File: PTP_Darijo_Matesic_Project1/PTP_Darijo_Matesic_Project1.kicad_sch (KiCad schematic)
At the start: 3 parts

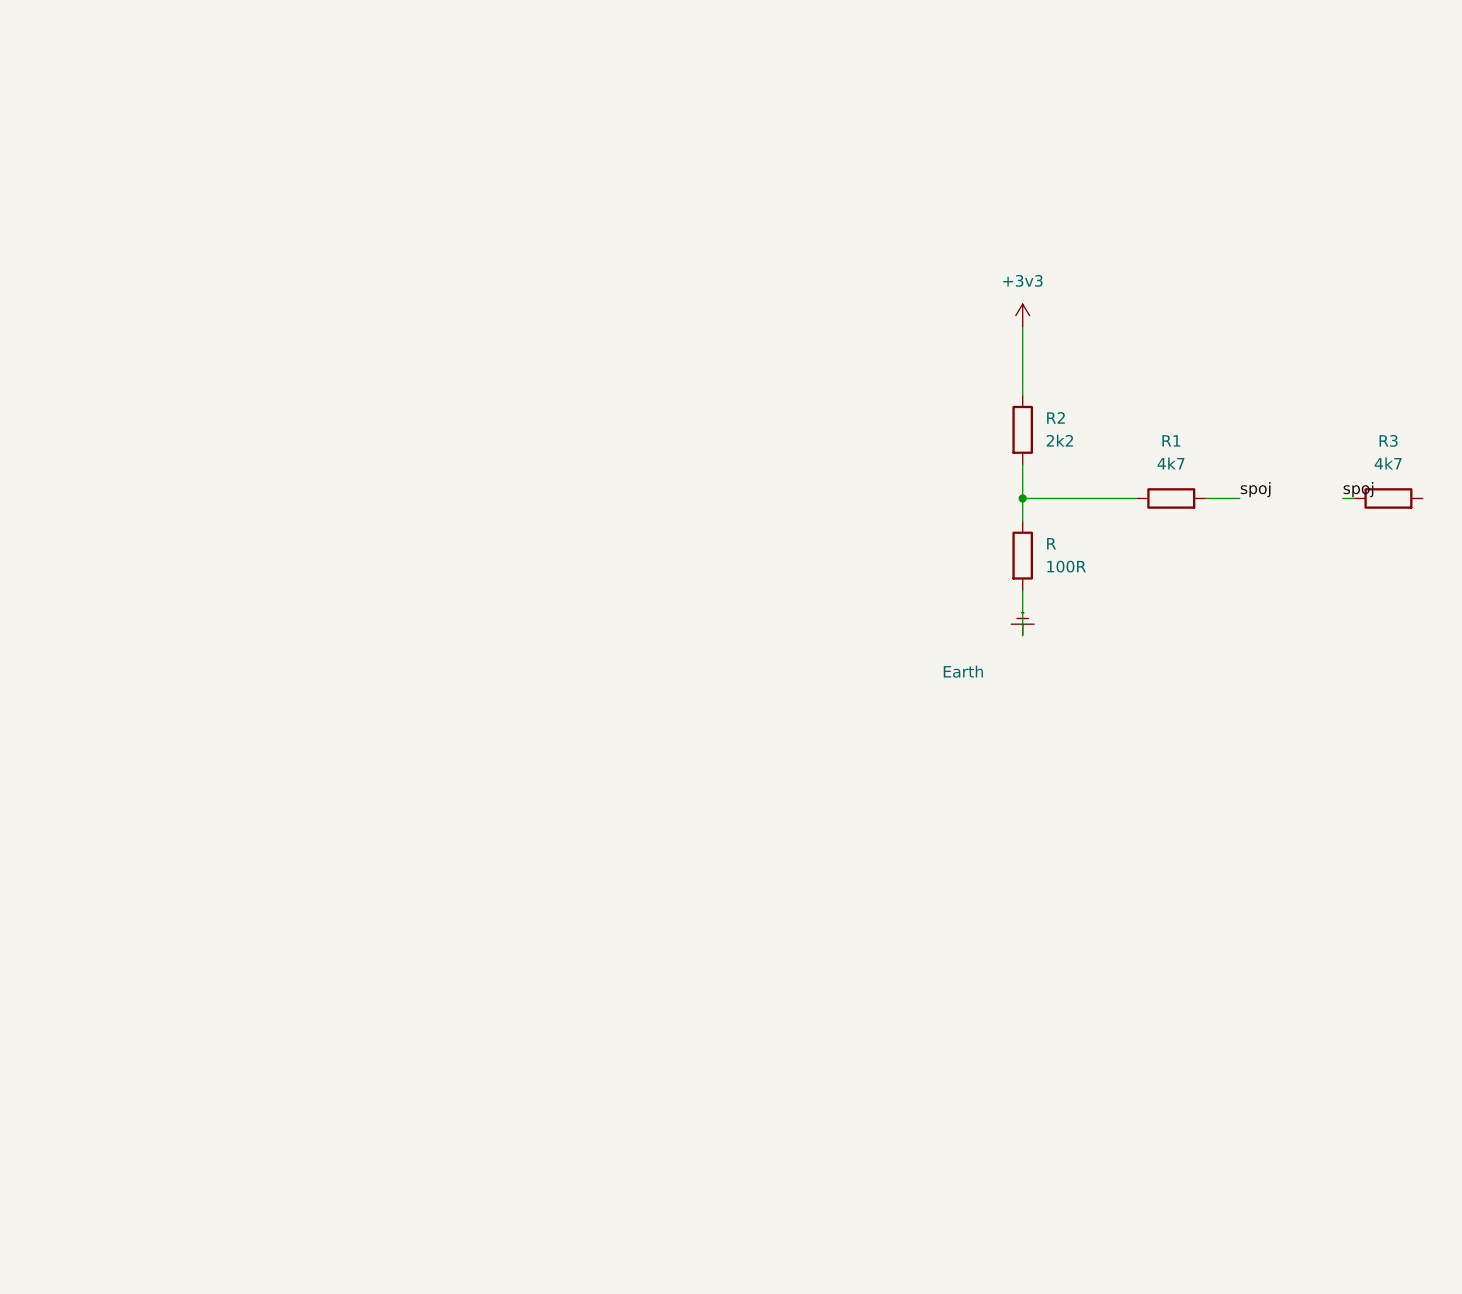
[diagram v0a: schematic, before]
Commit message: A
A
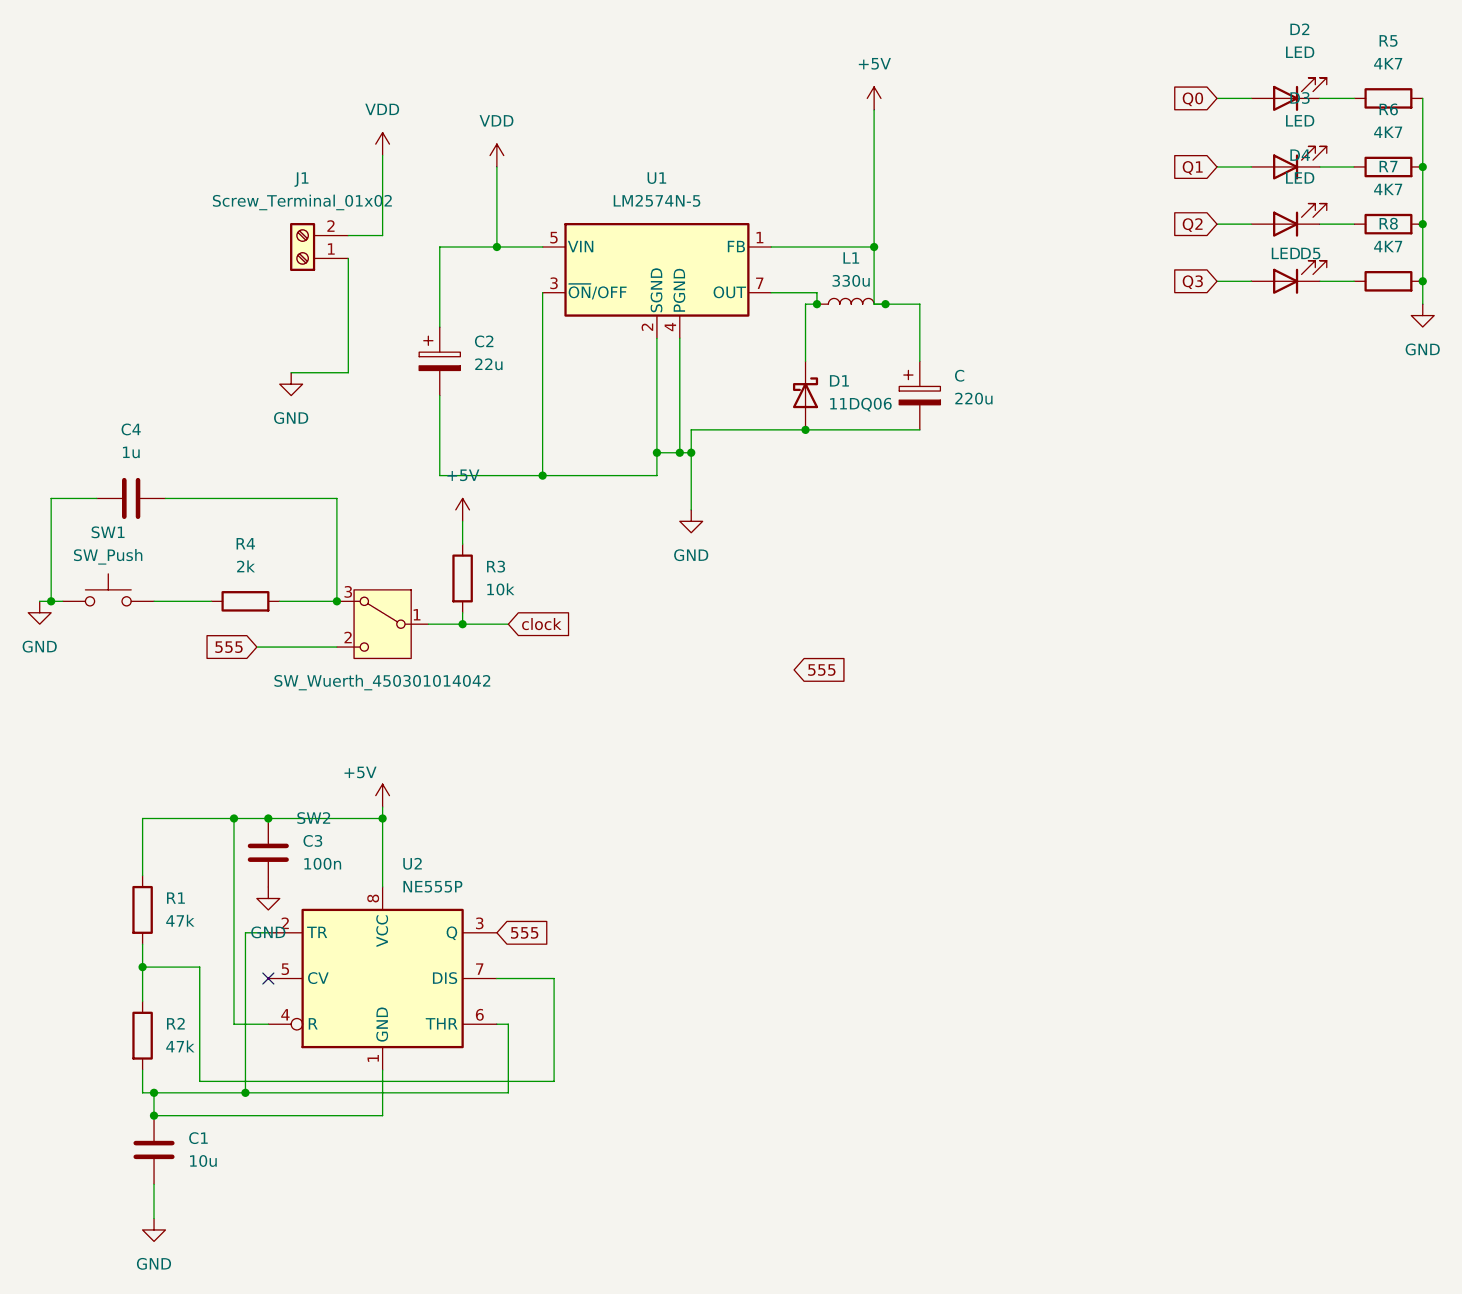
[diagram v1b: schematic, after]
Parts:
- added C: 220u, symbol Device:C_Polarized
- added C1: 10u, symbol Device:C
- added C2: 22u, symbol Device:C_Polarized
- added C3: 100n, symbol Device:C
- added C4: 1u, symbol Device:C
- added D1: 11DQ06, symbol Device:D_Schottky
- added D2, D3, D4, D5: LED, symbol Device:LED
- added J1: Screw_Terminal_01x02, symbol Connector:Screw_Terminal_01x02
- added L1: 330u, symbol Device:L
- added R4: 2k, symbol Device:R
- added R5, R6, R7, R8: 4K7, symbol Device:R
- added SW1: SW_Push, symbol Switch:SW_Push
- added SW2: SW_Wuerth_450301014042, Button_Switch_THT:SW_Slide-03_Wuerth-WS-SLTV_10x2.5x6.4_P2.54mm, symbol Switch:SW_Wuerth_450301014042
- added U1: LM2574N-5, Package_DIP:DIP-8_W7.62mm, symbol Regulator_Switching:LM2574N-5
- added U2: NE555P, Package_DIP:DIP-8_W7.62mm, symbol Timer:NE555P
- R1: value 4k7 -> 47k
- R2: value 2k2 -> 47k
- R3: value 4k7 -> 10k
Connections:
- net Earth is gone; now on an unnamed net: R1.2
- net at R2.2: now also C1.1, U2.1 (GND), U2.2 (TR), U2.6 (THR); no longer R1.1
- net clock: now reaches R3.2
- net clock: now also SW2.1 (B)
- net +3v3: no longer names the net of R2.1
- net +3v3: now also U2.7 (DIS)
- net spoj renamed +5V
- net +5V: now also R1.1, C.1, C3.1, L1.2, U1.1 (FB), U2.4 (R), U2.8 (VCC); no longer R1.2
- new net: C4.2, R4.2, SW2.3 (A)
- new net: D2.1 (K), R5.1
- new net: D4.1 (K), R7.1
- new net: D5.1 (K), R8.1
- new net: D1.1 (K), L1.1, U1.7 (OUT)
- new net: D3.1 (K), R6.1
- new net: R4.1, SW1.2
- new net 555: SW2.2 (C), U2.3 (Q)
- new net GND: C.2, C1.2, C2.2, C3.2, C4.1, D1.2 (A), J1.1 (Pin_1), R5.2, R6.2, R7.2, R8.2, SW1.1, U1.2 (SGND), U1.3 (~{ON}/OFF), U1.4 (PGND)
- new net Q0: D2.2 (A)
- new net Q1: D3.2 (A)
- new net Q2: D4.2 (A)
- new net Q3: D5.2 (A)
- new net VDD: C2.1, J1.2 (Pin_2), U1.5 (VIN)
- no-connect marks 0 -> 1
